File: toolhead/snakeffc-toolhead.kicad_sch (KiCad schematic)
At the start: 13 parts, among them J10 ZMIN, J11 SERVO, J12 E_STEPPER, J13 Conn_01x01, J14 Conn_01x01, J4 Conn_01x26, J5 HEATER_24V, J6 HEATER_SW, J7 THERMISTOR, J8 HOTEND_FAN, J9 PARTCOOLER_FAN, U2 ADXL345

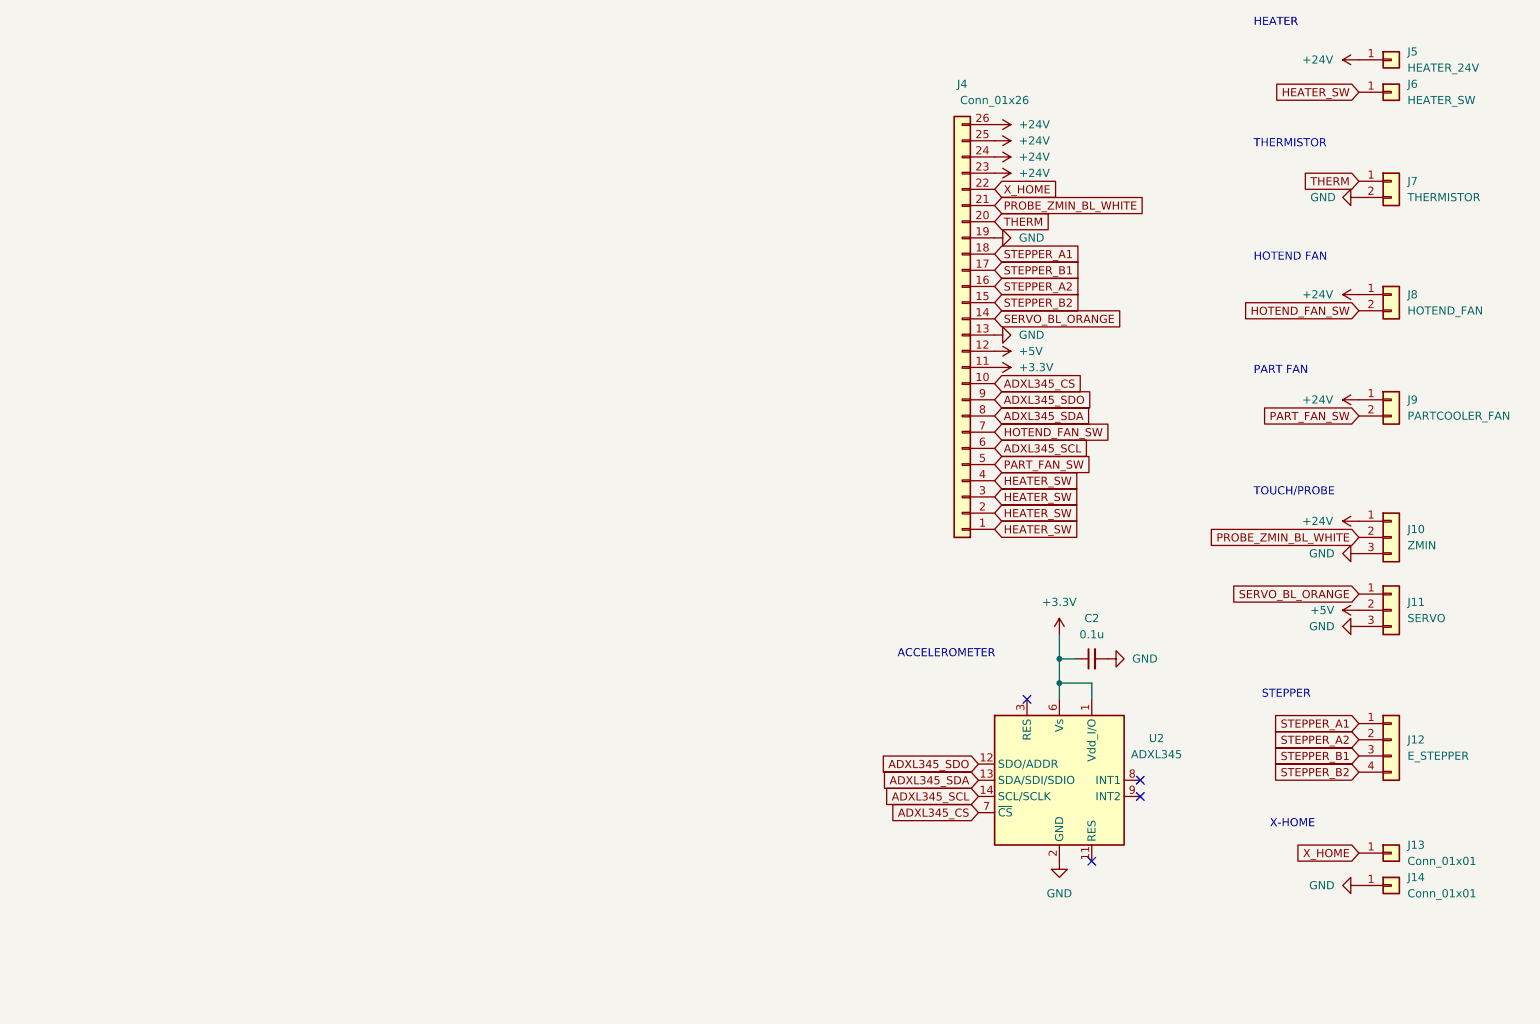
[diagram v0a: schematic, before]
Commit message: toolhead r3 schematic
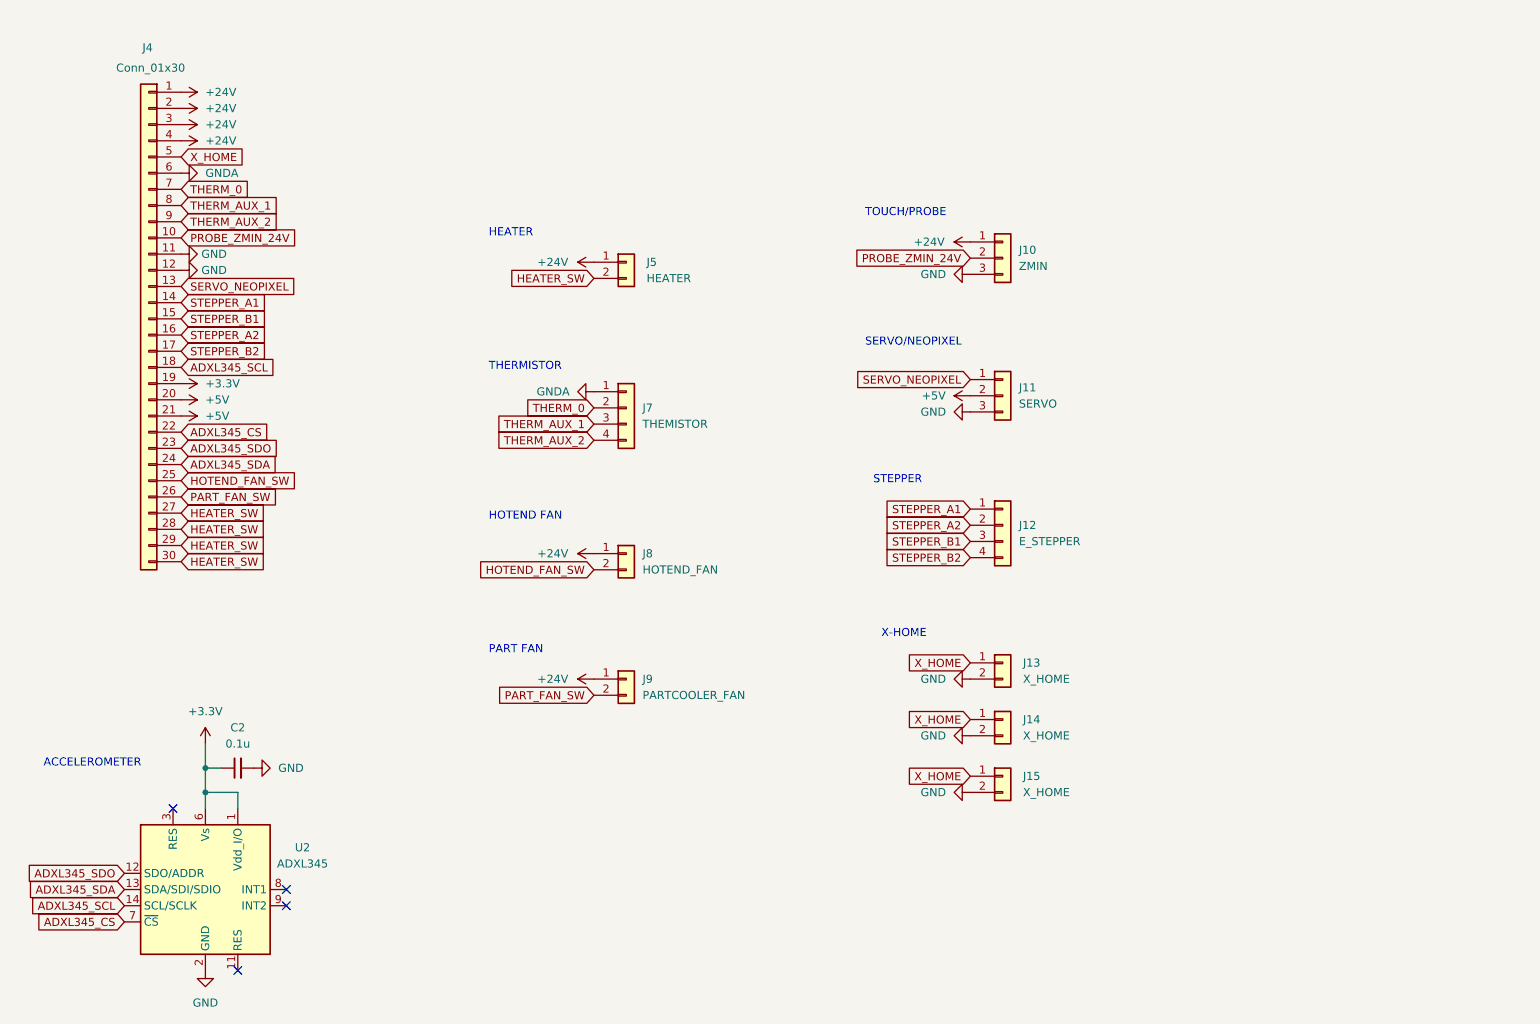
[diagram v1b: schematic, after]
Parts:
- removed J13, J14: Conn_01x01, Connector_PinHeader_2.54mm:PinHeader_1x01_P2.54mm_Vertical, symbol Connector_Generic:Conn_01x01
- removed J4: Conn_01x26, FFCconnector:FFC26pinTH, symbol Connector_Generic:Conn_01x26
- removed J5: HEATER_24V, Connector_Wire:SolderWire-2.5sqmm_1x01_D2.4mm_OD3.6mm, symbol Connector_Generic:Conn_01x01
- removed J6: HEATER_SW, Connector_Wire:SolderWire-2.5sqmm_1x01_D2.4mm_OD3.6mm, symbol Connector_Generic:Conn_01x01
- removed J7: THERMISTOR, Connector_PinHeader_2.54mm:PinHeader_1x02_P2.54mm_Vertical, symbol Connector_Generic:Conn_01x02
- added J13, J14, J15: X_HOME, Connector_PinHeader_2.54mm:PinHeader_1x02_P2.54mm_Vertical, symbol Connector_Generic:Conn_01x02
- added J4: Conn_01x30, ffc_connectors:ffc-30pin, symbol Connector_Generic:Conn_01x30
- added J5: HEATER, Connector_PinHeader_2.54mm:PinHeader_1x02_P2.54mm_Vertical, symbol Connector_Generic:Conn_01x02
- added J7: THEMISTOR, Connector_PinHeader_2.54mm:PinHeader_1x04_P2.54mm_Vertical, symbol Connector_Generic:Conn_01x04
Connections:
- net +24V: now also J4.1 (Pin_1), J4.2 (Pin_2), J4.3 (Pin_3), J4.4 (Pin_4), J5.1 (Pin_1)
- net +3V3: now also J4.19 (Pin_19)
- net +5V: now also J4.20 (Pin_20), J4.21 (Pin_21)
- net ADXL345_CS: now also J4.22 (Pin_22)
- net ADXL345_SCL: now also J4.18 (Pin_18)
- net ADXL345_SDA: now also J4.24 (Pin_24)
- net ADXL345_SDO: now also J4.23 (Pin_23)
- net GND: now also J13.2 (Pin_2), J14.2 (Pin_2), J15.2 (Pin_2), J4.11 (Pin_11), J4.12 (Pin_12)
- net HEATER_SW: now also J4.27 (Pin_27), J4.28 (Pin_28), J4.29 (Pin_29), J4.30 (Pin_30), J5.2 (Pin_2)
- net HOTEND_FAN_SW: now also J4.25 (Pin_25)
- net PART_FAN_SW: now also J4.26 (Pin_26)
- net STEPPER_A1: now also J4.14 (Pin_14)
- net STEPPER_A2: now also J4.16 (Pin_16)
- net STEPPER_B1: now also J4.15 (Pin_15)
- net STEPPER_B2: now also J4.17 (Pin_17)
- net X_HOME: now also J13.1 (Pin_1), J14.1 (Pin_1), J15.1 (Pin_1), J4.5 (Pin_5)
- net PROBE_ZMIN_BL_WHITE renamed PROBE_ZMIN_24V
- net PROBE_ZMIN_24V: now also J4.10 (Pin_10)
- net SERVO_BL_ORANGE renamed SERVO_NEOPIXEL
- net SERVO_NEOPIXEL: now also J4.13 (Pin_13)
- new net GNDA: J4.6 (Pin_6), J7.1 (Pin_1)
- new net THERM_0: J4.7 (Pin_7), J7.2 (Pin_2)
- new net THERM_AUX_1: J4.8 (Pin_8), J7.3 (Pin_3)
- new net THERM_AUX_2: J4.9 (Pin_9), J7.4 (Pin_4)
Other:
- note added: "SERVO/NEOPIXEL"
- moved on the sheet: C2, J10, J11, J12, J8, J9, U2
